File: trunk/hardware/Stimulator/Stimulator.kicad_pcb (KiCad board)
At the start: 2 copper layers, 58.4 x 31.8 mm, 101 parts, among them P1 CONN_1, P10 CONN_1, P11 CONN_1, P12 CONN_1, P13 CONN_1, P14 CONN_1, P15 CONN_1, P16 CONN_1, P17 CONN_1, P18 CONN_1, P19 CONN_1, P2 CONN_10X2, P20 CONN_1, P21 CONN_1, P22 CONN_1, P23 CONN_1, P24 CONN_1, P25 CONN_1, P26 CONN_1, P27 CONN_1, P28 CONN_1, P29 CONN_1, P3 CONN_1, P30 CONN_1, P31 CONN_1, P32 CONN_1, P33 CONN_1, P34 CONN_1, P35 CONN_1, P36 CONN_1, P37 CONN_10X2, P38 CONN_1, P39 CONN_1, P4 CONN_1, P40 CONN_1, P41 CONN_1, P42 CONN_1, P43 CONN_1, P44 CONN_1, P45 CONN_1, P46 CONN_1, P47 CONN_1, P48 CONN_1, P49 CONN_1, P5 CONN_1, P50 CONN_1, P51 CONN_1, P52 CONN_1, P53 CONN_1, P54 CONN_1, P55 CONN_1, P56 CONN_1, P57 CONN_1, P6 CONN_1, P7 CONN_1, P8 CONN_1, P9 CONN_1, Q1 2N7002, Q2 2N7002, Q3 2N7002, Q4 2N7002, U1 MCP42010, U2 MCP42010, U3 MCP42010, U4 MCP42010

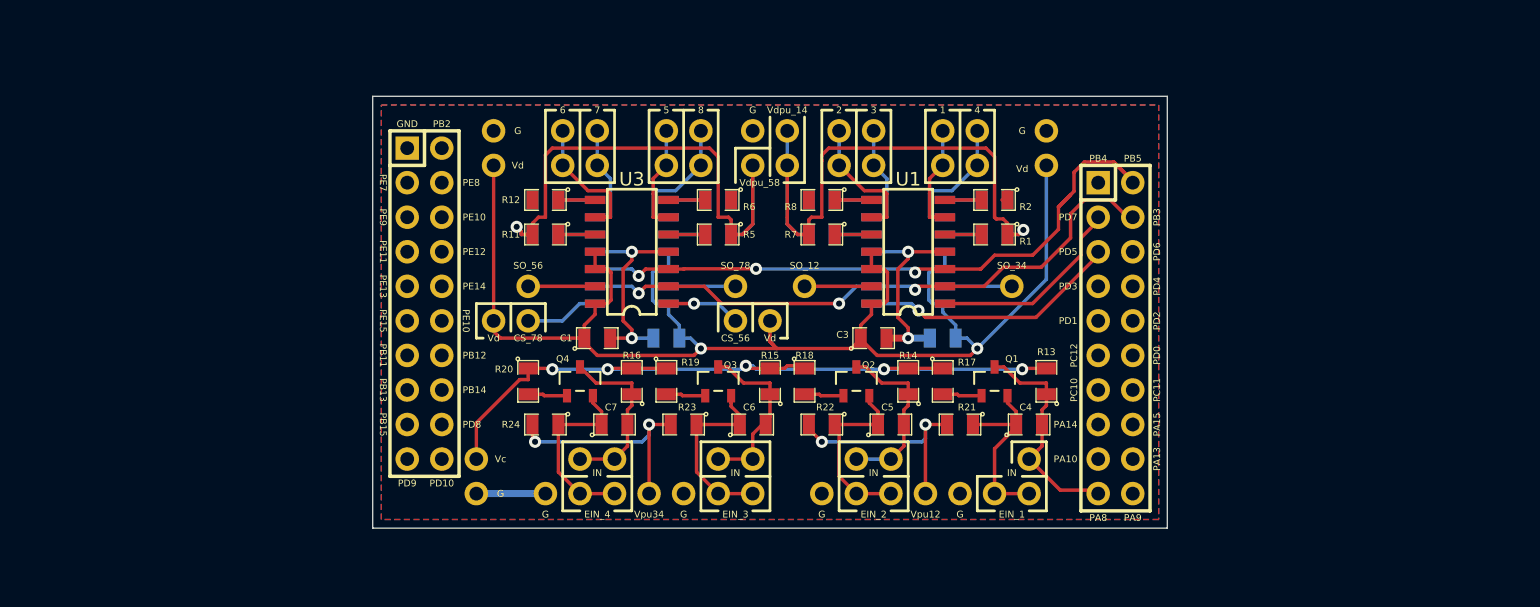
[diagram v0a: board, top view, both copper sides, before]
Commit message: 2N7002KCT-ND
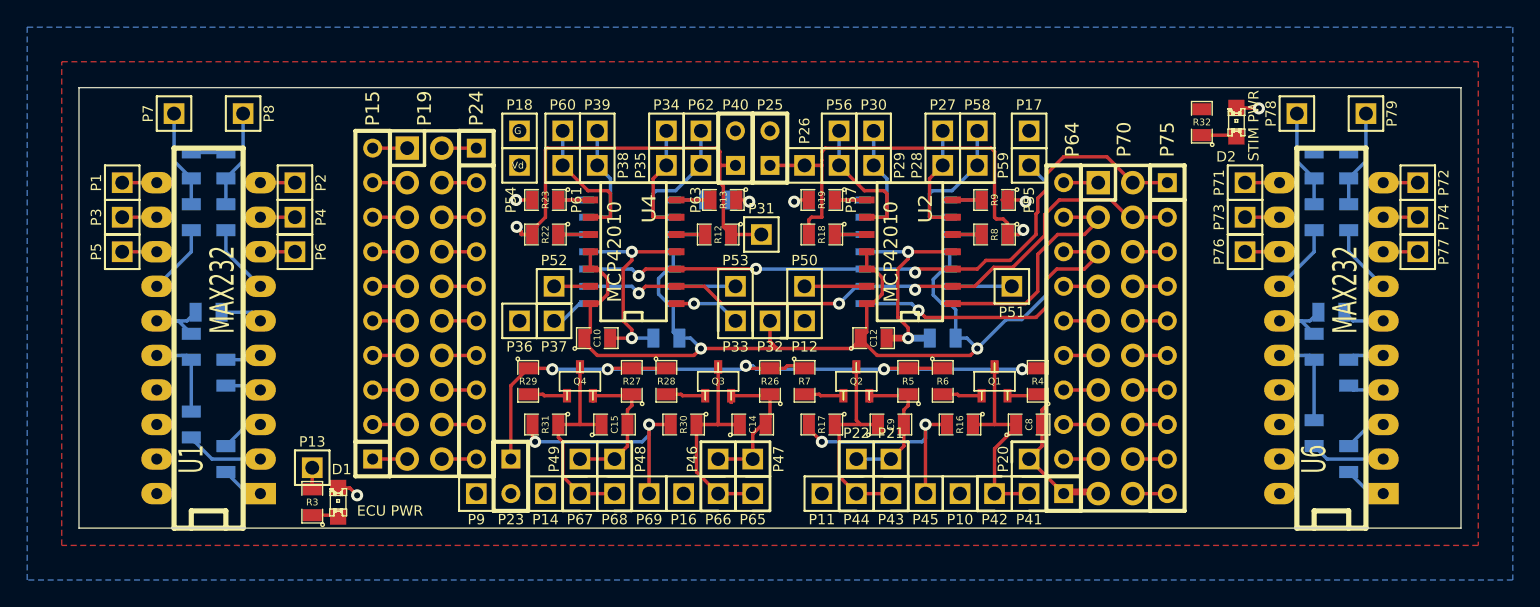
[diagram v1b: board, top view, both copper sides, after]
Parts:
- added C1: 1uF, SM0805, B.Cu at (111.1, 85.1)
- added C16: 1uF, SM0805, B.Cu at (193.7, 85.1)
- added C17: 1uF, SM0805, B.Cu at (193.7, 78.7)
- added C18: 1uF, SM0805, B.Cu at (191.1, 83.2)
- added C19: 1uF, SM0805, B.Cu at (192.4, 74.3)
- added C2: 1uF, SM0805, B.Cu at (111.1, 78.7)
- added C20: 1uF, SM0805, B.Cu at (191.1, 76.8)
- added C21: 1uF, SM0805, B.Cu at (191.1, 67.3)
- added C22: 1uF, SM0805, B.Cu at (193.7, 67.3)
- added C3: 1uF, SM0805, B.Cu at (108.6, 82.5)
- added C4: 1uF, SM0805, B.Cu at (109.9, 74.3)
- added C5: 1uF, SM0805, B.Cu at (108.6, 76.8)
- added C6: 1uF, SM0805, B.Cu at (108.6, 67.3)
- added C7: 1uF, SM0805, B.Cu at (111.1, 67.3)
- added D1: ECU PWR, LED-0805, F.Cu at (119.4, 88.3)
- added D2: STIM PWR, LED-0805, F.Cu at (185.4, 60.3)
- added P1: CONN_1, PIN_ARRAY_1, F.Cu at (103.5, 64.8)
- added P13: CONN_1, PIN_ARRAY_1, F.Cu at (117.5, 85.7)
- added P15: CONN_10, SIL-10, F.Cu at (121.9, 73.7)
- added P2: CONN_1, PIN_ARRAY_1, F.Cu at (116.2, 64.8)
- added P24: CONN_10, SIL-10, F.Cu at (129.5, 73.7)
- added P3: CONN_1, PIN_ARRAY_1, F.Cu at (103.5, 67.3)
- added P4: CONN_1, PIN_ARRAY_1, F.Cu at (116.2, 67.3)
- added P40: TEST, SIL-2, F.Cu at (148.6, 62.2)
- added P5: CONN_1, PIN_ARRAY_1, F.Cu at (103.5, 69.8)
- added P6: CONN_1, PIN_ARRAY_1, F.Cu at (116.2, 69.8)
- added P64: CONN_10, SIL-10, F.Cu at (172.7, 76.2)
- added P7: CONN_1, PIN_ARRAY_1, F.Cu at (107.3, 59.7)
- added P71: CONN_1, PIN_ARRAY_1, F.Cu at (186.1, 64.8)
- added P72: CONN_1, PIN_ARRAY_1, F.Cu at (198.8, 64.8)
- added P73: CONN_1, PIN_ARRAY_1, F.Cu at (186.1, 67.3)
- added P74: CONN_1, PIN_ARRAY_1, F.Cu at (198.8, 67.3)
- added P75: CONN_10, SIL-10, F.Cu at (180.3, 76.2)
- added P76: CONN_1, PIN_ARRAY_1, F.Cu at (186.1, 69.8)
- added P77: CONN_1, PIN_ARRAY_1, F.Cu at (198.8, 69.8)
- added P78: CONN_1, PIN_ARRAY_1, F.Cu at (189.9, 59.7)
- added P79: CONN_1, PIN_ARRAY_1, F.Cu at (194.9, 59.7)
- added P8: CONN_1, PIN_ARRAY_1, F.Cu at (112.4, 59.7)
- added R1: 10k, SM0805, B.Cu at (108.6, 63.5)
- added R2: 10k, SM0805, B.Cu at (111.1, 63.5)
- added R3: 700R, SM0805, F.Cu at (117.5, 88.3)
- added R32: 700R, SM0805, F.Cu at (182.9, 60.3)
- added R33: 10k, SM0805, B.Cu at (191.1, 63.5)
- added R34: 10k, SM0805, B.Cu at (193.7, 63.5)
- added U1: MAX232, DIP-20__300_ELL, F.Cu at (109.9, 76.2)
- added U6: MAX232, DIP-20__300_ELL, F.Cu at (192.4, 76.2)
- C10: renamed from C1; footprint SMD_Packages:SM0805 -> SM0805
- C11: renamed from C2; footprint SMD_Packages:SM0805 -> SM0805
- C12: renamed from C3; footprint SMD_Packages:SM0805 -> SM0805
- C13: renamed from C8; footprint SMD_Packages:SM0805 -> SM0805
- C14: renamed from C6; footprint SMD_Packages:SM0805 -> SM0805
- C15: renamed from C7; footprint SMD_Packages:SM0805 -> SM0805
- C8: renamed from C4; footprint SMD_Packages:SM0805 -> SM0805
- C9: renamed from C5; footprint SMD_Packages:SM0805 -> SM0805
- P10: renamed from P39; footprint Stimulator:1PIN_A -> PIN_ARRAY_1
- P11: renamed from P40; footprint Stimulator:1PIN_A -> PIN_ARRAY_1
- P12: renamed from P41; footprint Stimulator:1PIN_A -> PIN_ARRAY_1
- P14: renamed from P42; footprint Stimulator:1PIN_A -> PIN_ARRAY_1
- P16: renamed from P43; footprint Stimulator:1PIN_A -> PIN_ARRAY_1
- P17: renamed from P44; footprint Stimulator:1PIN_A -> PIN_ARRAY_1
- P18: renamed from P1; footprint Stimulator:1PIN_A -> PIN_ARRAY_1
- P20, P21, P22: footprint Stimulator:1PIN_A -> PIN_ARRAY_1
- P23: renamed from P27; value CONN_1 -> TEST; footprint Stimulator:1PIN_A -> SIL-2
- P25: renamed from P57; value CONN_1 -> TEST; footprint Stimulator:1PIN_A -> SIL-2
- P26: renamed from P3; footprint Stimulator:1PIN_A -> PIN_ARRAY_1
- P27: renamed from P4; footprint Stimulator:1PIN_A -> PIN_ARRAY_1
- P28: renamed from P5; footprint Stimulator:1PIN_A -> PIN_ARRAY_1
- P29: renamed from P6; footprint Stimulator:1PIN_A -> PIN_ARRAY_1
- P30: renamed from P7; footprint Stimulator:1PIN_A -> PIN_ARRAY_1
- P31: renamed from P52; footprint Stimulator:1PIN_A -> PIN_ARRAY_1
- P32: renamed from P55; footprint Stimulator:1PIN_A -> PIN_ARRAY_1
- P33: renamed from P45; footprint Stimulator:1PIN_A -> PIN_ARRAY_1
- P34: renamed from P8; footprint Stimulator:1PIN_A -> PIN_ARRAY_1
- P35: renamed from P9; footprint Stimulator:1PIN_A -> PIN_ARRAY_1
- P36: renamed from P56; footprint Stimulator:1PIN_A -> PIN_ARRAY_1
- P37: renamed from P46; footprint Stimulator:1PIN_A -> PIN_ARRAY_1
- P38: renamed from P47; footprint Stimulator:1PIN_A -> PIN_ARRAY_1
- P39: renamed from P48; footprint Stimulator:1PIN_A -> PIN_ARRAY_1
- P41: renamed from P28; footprint Stimulator:1PIN_A -> PIN_ARRAY_1
- P42: renamed from P29; footprint Stimulator:1PIN_A -> PIN_ARRAY_1
- P43: renamed from P30; footprint Stimulator:1PIN_A -> PIN_ARRAY_1
- P44: renamed from P31; footprint Stimulator:1PIN_A -> PIN_ARRAY_1
- P45: renamed from P36; footprint Stimulator:1PIN_A -> PIN_ARRAY_1
- P46: renamed from P23; footprint Stimulator:1PIN_A -> PIN_ARRAY_1
- P47: renamed from P24; footprint Stimulator:1PIN_A -> PIN_ARRAY_1
- P48: renamed from P25; footprint Stimulator:1PIN_A -> PIN_ARRAY_1
- P49: renamed from P26; footprint Stimulator:1PIN_A -> PIN_ARRAY_1
- P50: renamed from P10; footprint Stimulator:1PIN_A -> PIN_ARRAY_1
- P51: renamed from P11; footprint Stimulator:1PIN_A -> PIN_ARRAY_1
- P52: renamed from P12; footprint Stimulator:1PIN_A -> PIN_ARRAY_1
- P53: renamed from P49; footprint Stimulator:1PIN_A -> PIN_ARRAY_1
- P54: renamed from P13; footprint Stimulator:1PIN_A -> PIN_ARRAY_1
- P55: renamed from P53; footprint Stimulator:1PIN_A -> PIN_ARRAY_1
- P56: renamed from P14; footprint Stimulator:1PIN_A -> PIN_ARRAY_1
- P57: renamed from P15; footprint Stimulator:1PIN_A -> PIN_ARRAY_1
- P58: renamed from P16; footprint Stimulator:1PIN_A -> PIN_ARRAY_1
- P59: renamed from P17; footprint Stimulator:1PIN_A -> PIN_ARRAY_1
- P60: renamed from P18; footprint Stimulator:1PIN_A -> PIN_ARRAY_1
- P61: renamed from P19; footprint Stimulator:1PIN_A -> PIN_ARRAY_1
- P62: renamed from P50; footprint Stimulator:1PIN_A -> PIN_ARRAY_1
- P63: renamed from P51; footprint Stimulator:1PIN_A -> PIN_ARRAY_1
- P65: renamed from P32; footprint Stimulator:1PIN_A -> PIN_ARRAY_1
- P66: renamed from P33; footprint Stimulator:1PIN_A -> PIN_ARRAY_1
- P67: renamed from P34; footprint Stimulator:1PIN_A -> PIN_ARRAY_1
- P68: renamed from P35; footprint Stimulator:1PIN_A -> PIN_ARRAY_1
- P69: renamed from P54; footprint Stimulator:1PIN_A -> PIN_ARRAY_1
- P9: renamed from P38; footprint Stimulator:1PIN_A -> PIN_ARRAY_1
- Q1, Q2, Q3, Q4: footprint Transistors_SMD:sot23 -> sot23
- R10: renamed from R3; footprint SMD_Packages:SM0805 -> SM0805
- R11: renamed from R4; footprint SMD_Packages:SM0805 -> SM0805
- R12: renamed from R5; footprint SMD_Packages:SM0805 -> SM0805
- R13: renamed from R6; footprint SMD_Packages:SM0805 -> SM0805
- R14: renamed from R25; footprint SMD_Packages:SM0805 -> SM0805
- R15: renamed from R26; footprint SMD_Packages:SM0805 -> SM0805
- R16: renamed from R21; footprint SMD_Packages:SM0805 -> SM0805
- R17: renamed from R22; footprint SMD_Packages:SM0805 -> SM0805
- R18: renamed from R7; footprint SMD_Packages:SM0805 -> SM0805
- R19: renamed from R8; footprint SMD_Packages:SM0805 -> SM0805
- R20: renamed from R9; footprint SMD_Packages:SM0805 -> SM0805
- R21: renamed from R10; footprint SMD_Packages:SM0805 -> SM0805
- R22: renamed from R11; footprint SMD_Packages:SM0805 -> SM0805
- R23: renamed from R12; footprint SMD_Packages:SM0805 -> SM0805
- R24: renamed from R27; footprint SMD_Packages:SM0805 -> SM0805
- R25: renamed from R28; footprint SMD_Packages:SM0805 -> SM0805
- R26: renamed from R15; footprint SMD_Packages:SM0805 -> SM0805
- R27: renamed from R16; footprint SMD_Packages:SM0805 -> SM0805
- R28: renamed from R19; footprint SMD_Packages:SM0805 -> SM0805
- R29: renamed from R20; footprint SMD_Packages:SM0805 -> SM0805
- R30: renamed from R23; footprint SMD_Packages:SM0805 -> SM0805
- R31: renamed from R24; footprint SMD_Packages:SM0805 -> SM0805
- R4: renamed from R13; footprint SMD_Packages:SM0805 -> SM0805
- R5: renamed from R14; footprint SMD_Packages:SM0805 -> SM0805
- R6: renamed from R17; footprint SMD_Packages:SM0805 -> SM0805
- R7: renamed from R18; footprint SMD_Packages:SM0805 -> SM0805
- R8: renamed from R1; footprint SMD_Packages:SM0805 -> SM0805
- R9: renamed from R2; footprint SMD_Packages:SM0805 -> SM0805
- U2: renamed from U1; footprint SOIC_Packages:SOIC-14_Narrow -> SO14N
- U3: renamed from U2; footprint SOIC_Packages:SOIC-14_Narrow -> SO14N
- U4: renamed from U3; footprint SOIC_Packages:SOIC-14_Narrow -> SO14N
- U5: renamed from U4; footprint SOIC_Packages:SOIC-14_Narrow -> SO14N
- moved P12 14.5 mm to (153.7, 74.9), turned to 180 degrees
- moved P31 5.12 mm to (150.5, 68.6)
- moved P23 2.84 mm to (132.1, 86.4), turned to 270 degrees
- moved P18 1.91 mm to (132.7, 61.0), turned to 0 degrees
- moved P36 1.91 mm to (132.7, 74.9), turned to 180 degrees
- moved P37 1.91 mm to (135.3, 74.9), turned to 180 degrees
- moved P52 1.91 mm to (135.3, 72.4)
- moved P54 1.91 mm to (132.7, 63.5)
- moved P25 1.80 mm to (151.1, 62.2), turned to 90 degrees
- moved P17 1.27 mm to (170.2, 61.0)
- moved P26 1.27 mm to (153.7, 63.5), turned to 270 degrees
- moved P55 1.27 mm to (170.2, 63.5), turned to 270 degrees
- moved R4 0.63 mm to (170.8, 79.4)
- moved R13 0.38 mm to (147.7, 66.0)
- turned P10 to 180 degrees
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- renumbered P2 to P19, P37 to P70
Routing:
- net GND: track 40.3 -> 59.5 mm, vias 4 -> 10
- net /Vdpu_14: track 44.4 -> 33.0 mm
- net /Vdpu_58: track 42.3 -> 32.5 mm
- net /Vd: track 109.2 -> 100.3 mm
- net N-0000052: track 0.00 -> 7.19 mm
- net N-0000050: track 0.00 -> 7.19 mm
- net N-0000056: track 0.00 -> 7.19 mm
- net N-0000055: track 0.00 -> 7.19 mm
- net N-0000074: track 0.00 -> 5.77 mm
- net N-0000039: track 0.00 -> 5.47 mm
- net N-0000051: track 0.00 -> 5.18 mm
- net N-0000057: track 0.00 -> 5.18 mm
- net N-0000053: track 0.00 -> 5.18 mm
- net N-0000043: track 0.00 -> 5.18 mm
- net /MOSI: track 52.8 -> 48.5 mm
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- added copper zone on F.Cu, net /Vd
- removed copper zone on F.Cu, net GND
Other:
- board size 58.4 x 31.8 mm -> 101.6 x 32.4 mm
- board text added: "DanMoto Stimulator June 2014 R0.2"
- board text removed: "DanMoto Stimulator June 2014"
